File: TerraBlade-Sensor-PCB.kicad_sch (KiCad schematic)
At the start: 25 parts, among them SW1 TS-1187A-B-A-B, U1 XIAO-ESP32-C3-SMD, U2 2.1MHz

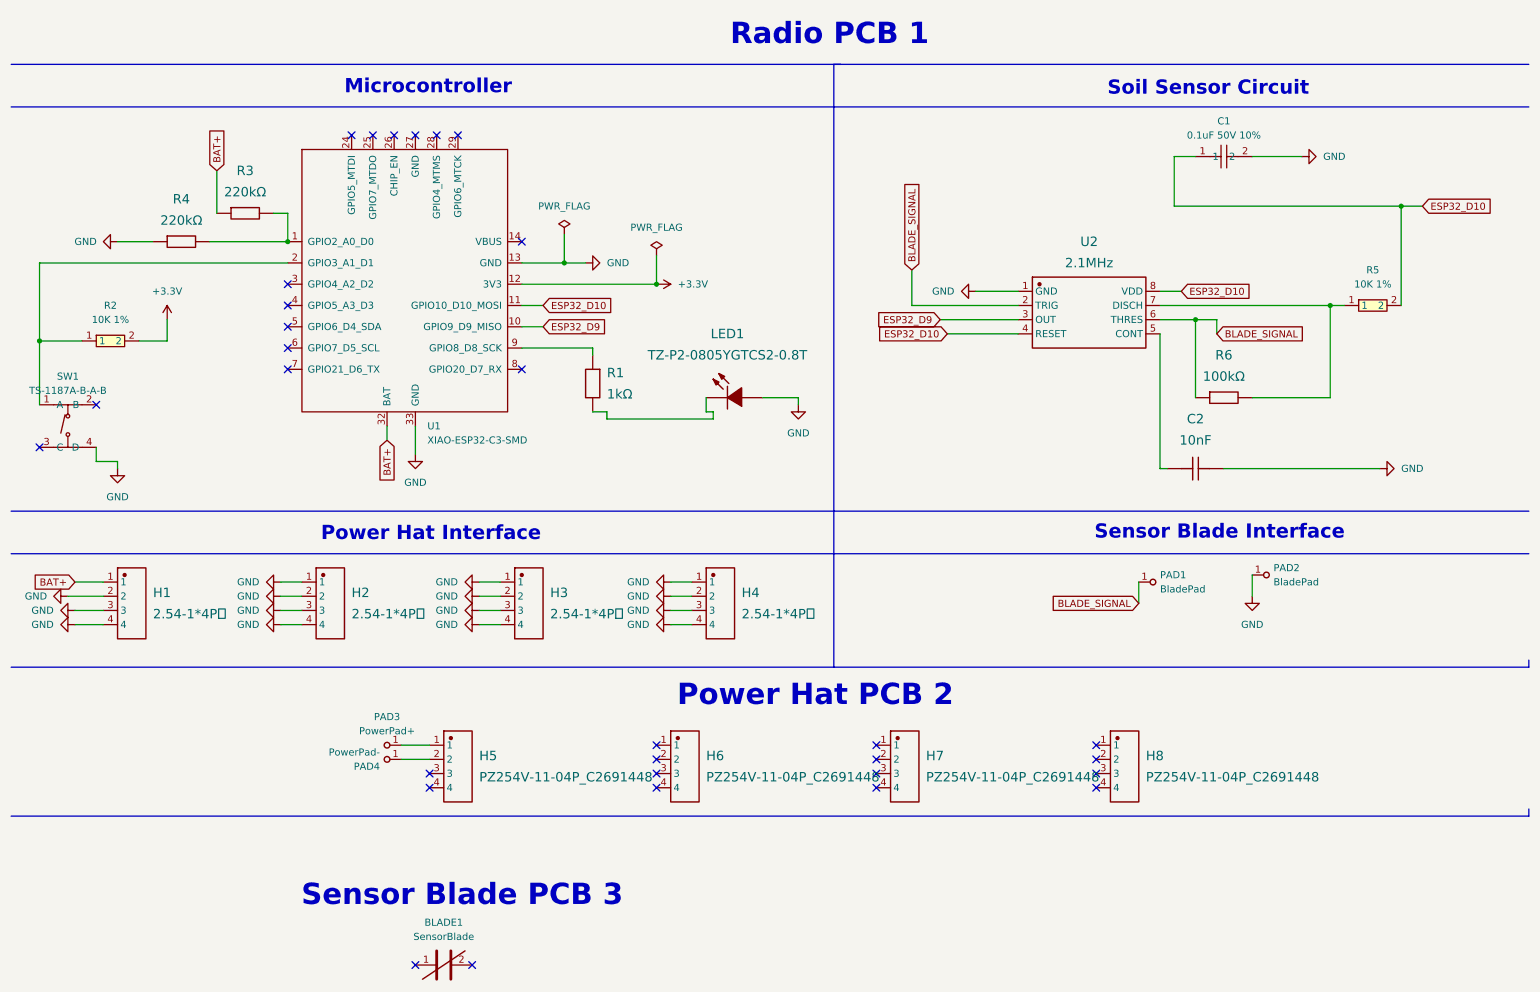
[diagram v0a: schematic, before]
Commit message: PCB Design
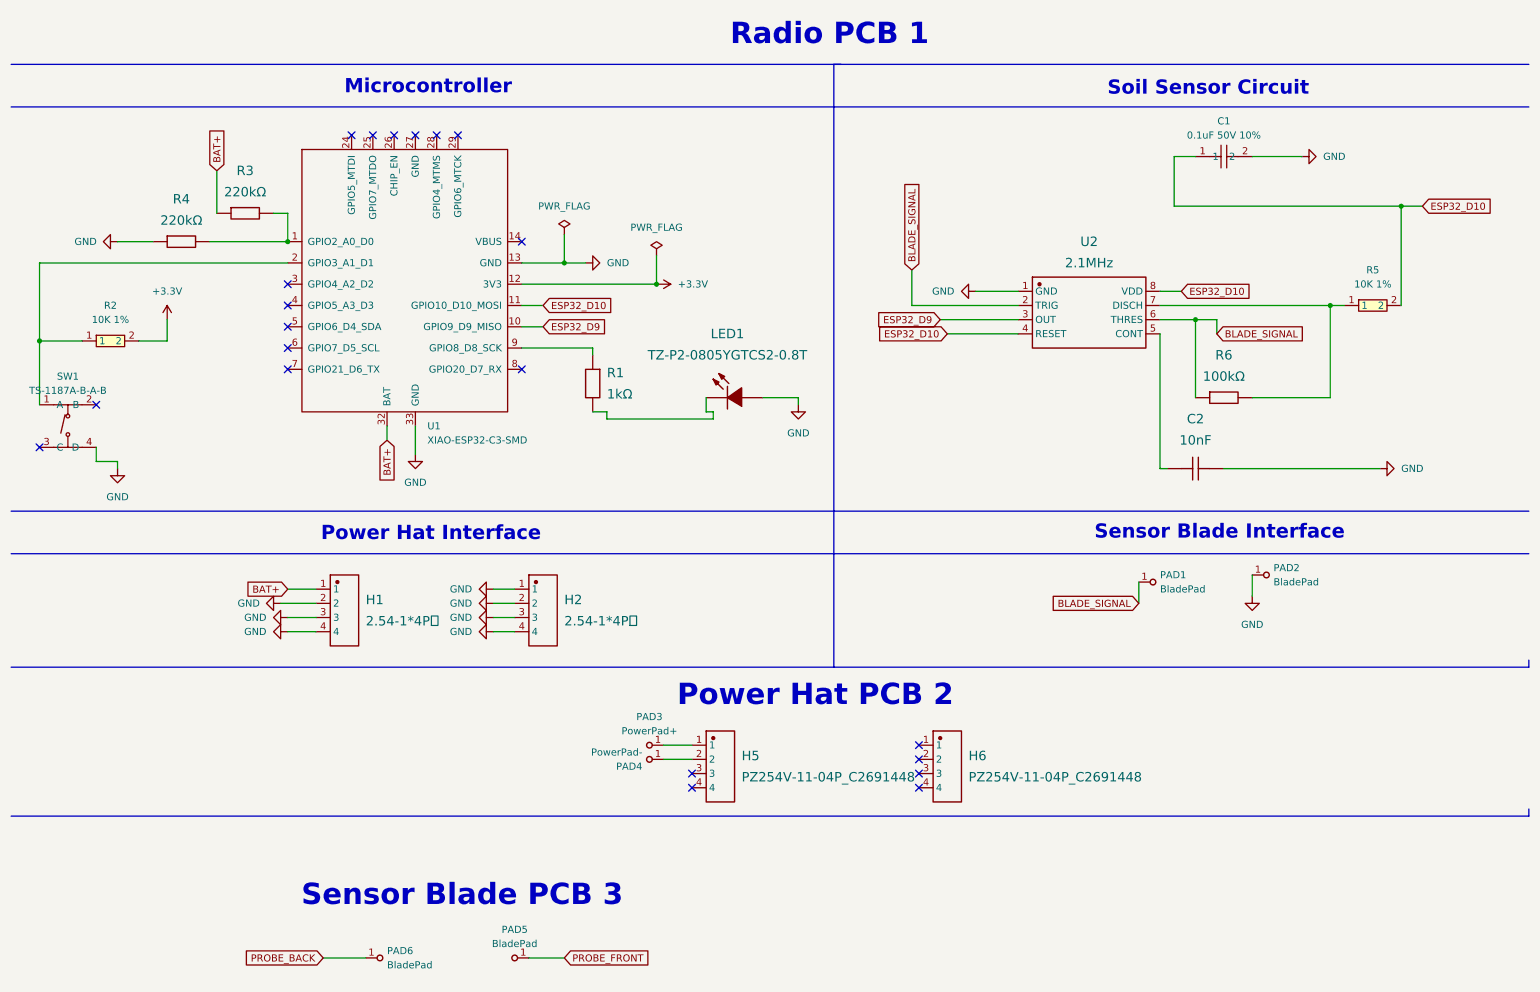
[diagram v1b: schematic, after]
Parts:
- removed BLADE1: SensorBlade, SensorBlade:SensorBlade_Tenon, symbol SensorBlade:SensorBlade
- removed H3, H4: 2.54-1*4P母, Custom:HDR-TH_4P-P2.54-V-F, symbol Custom:2.54-1*4P母
- removed H7, H8: PZ254V-11-04P_C2691448, Custom:HDR-TH_4P-P2.54-V-M, symbol Custom:PZ254V-11-04P_C2691448
- added PAD5, PAD6: BladePad, Custom:BladePad_SMD, symbol Custom:BladePad
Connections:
- new net PROBE_BACK: PAD6.1
- new net PROBE_FRONT: PAD5.1
- no-connect marks 31 -> 21
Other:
- moved on the sheet: H1, H2, H5, H6, PAD3, PAD4

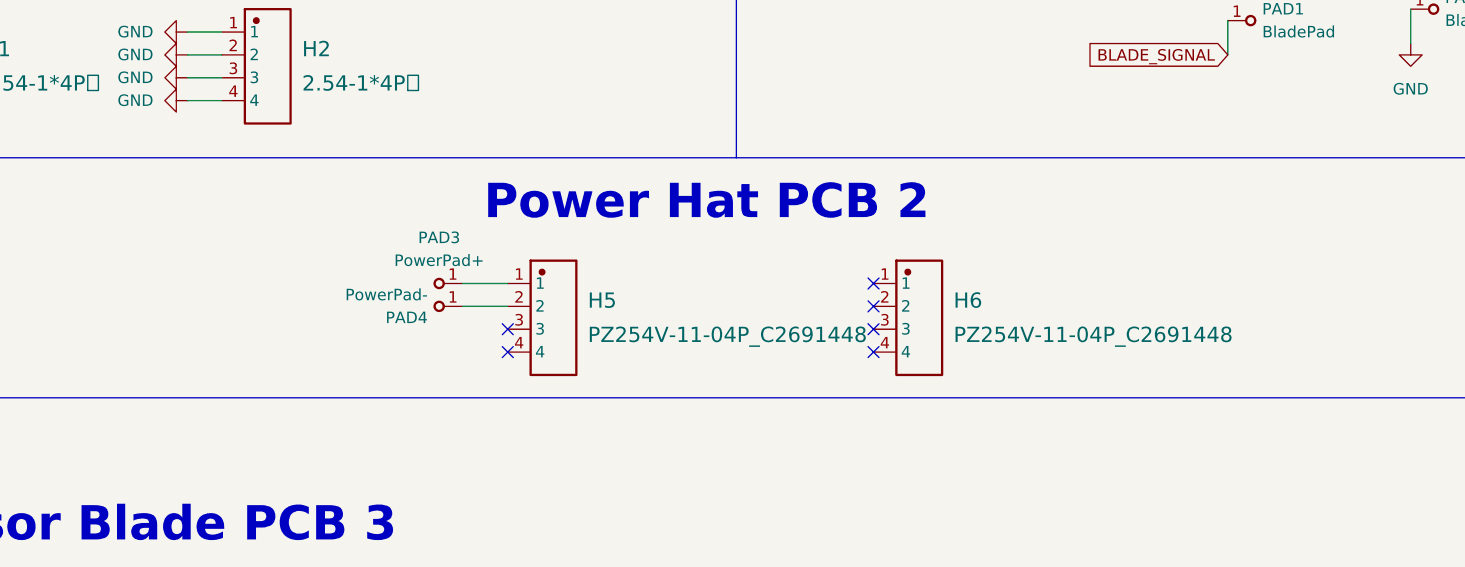
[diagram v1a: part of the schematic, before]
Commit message: PCB Layout
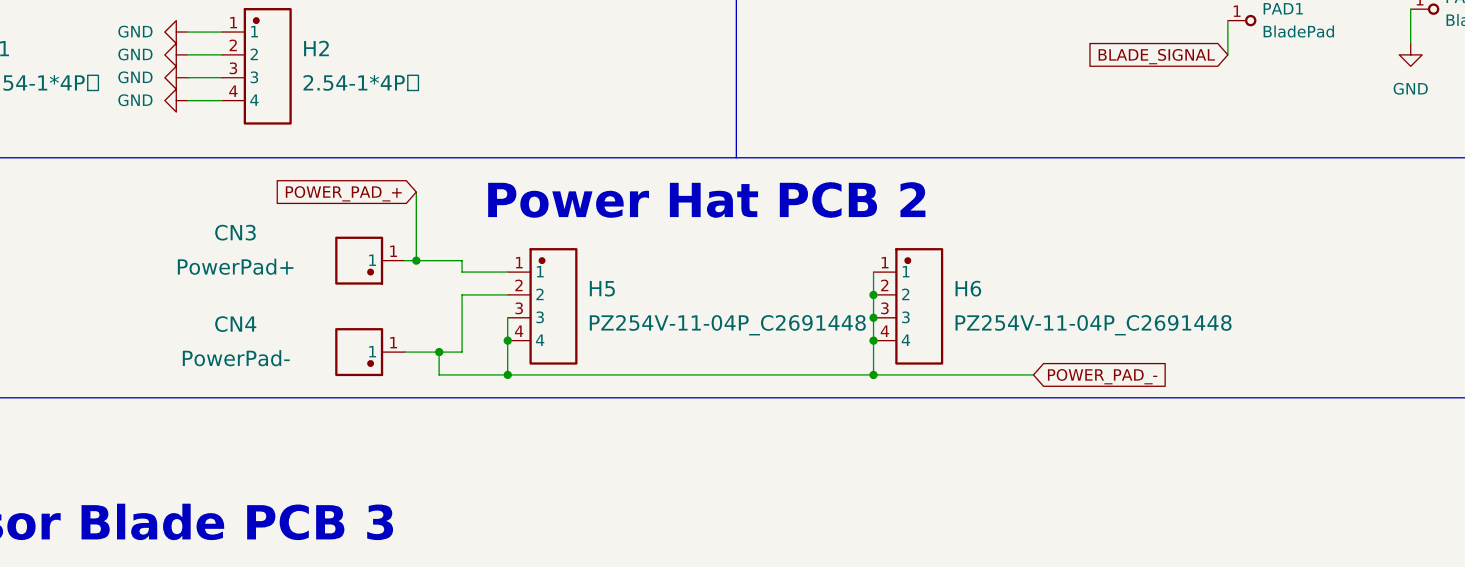
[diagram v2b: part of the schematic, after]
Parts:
- removed PAD3: PowerPad+, Custom:BladePad_SMD, symbol Custom:BladePad
- removed PAD4: PowerPad-, Custom:BladePad_SMD, symbol Custom:BladePad
- added CN3: PowerPad+, Custom:TESTPOINT-SMD_BD2.0-D1.0-Custom, symbol Custom:PG1000-01-010P
- added CN4: PowerPad-, Custom:TESTPOINT-SMD_BD2.0-D1.0-Custom, symbol Custom:PG1000-01-010P
- C1: Supplier Part (none) -> C476766
- R2, R5: Supplier Part (none) -> C17414
- SW1: Supplier Part (none) -> C318884
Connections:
- net POWER_PAD_+: now reaches H5.1
- net POWER_PAD_+: now also CN3.1
- net POWER_PAD_-: now reaches H5.2
- net POWER_PAD_-: now also H5.3, H5.4, H6.1, H6.2, H6.3, H6.4, CN4.1
- no-connect marks 21 -> 15
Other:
- moved on the sheet: H5, H6
